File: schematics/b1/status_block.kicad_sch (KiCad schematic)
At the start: 22 parts, among them Q1 2N3904, SW5 SW_SPDT, U4 74HC595

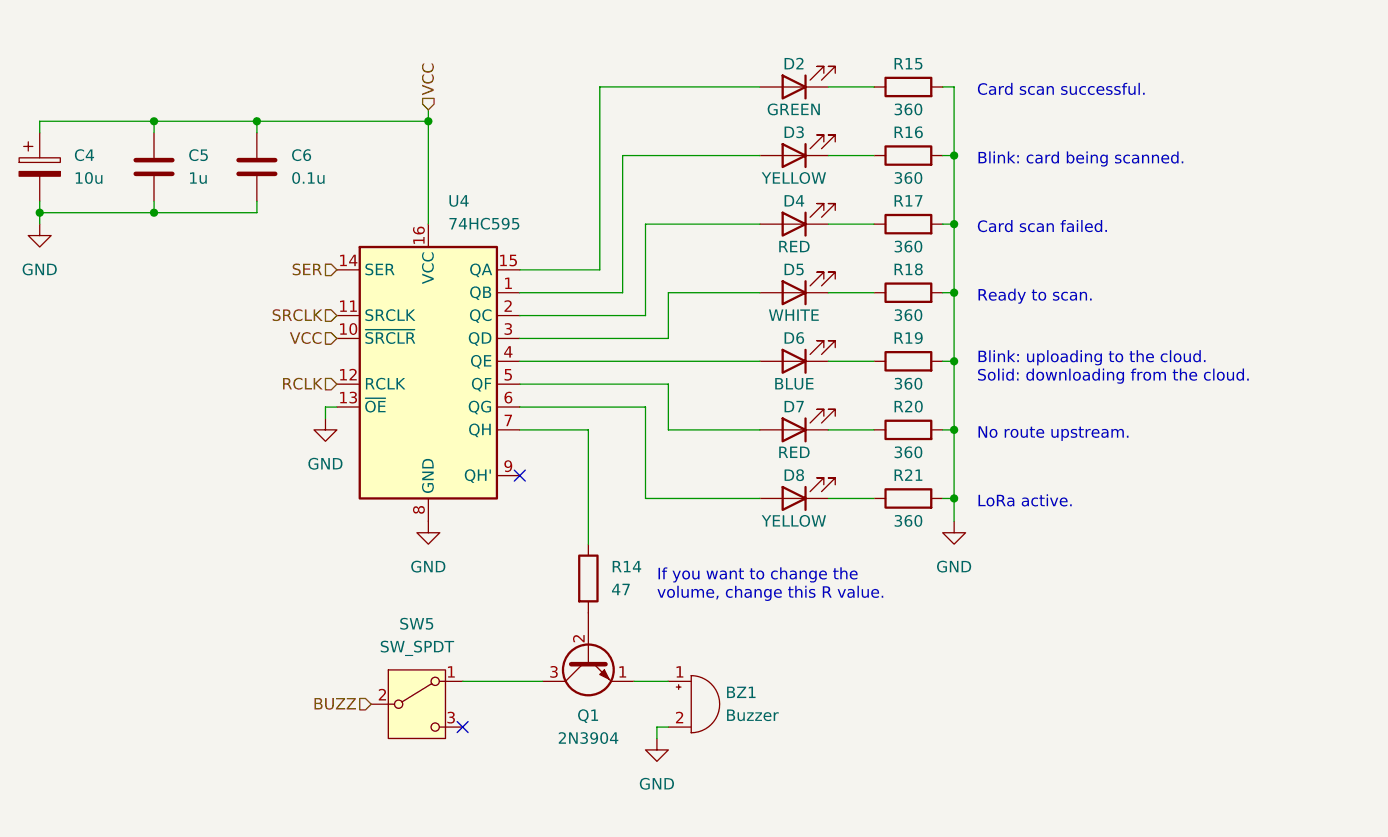
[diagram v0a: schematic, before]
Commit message: Updated buzz switch.
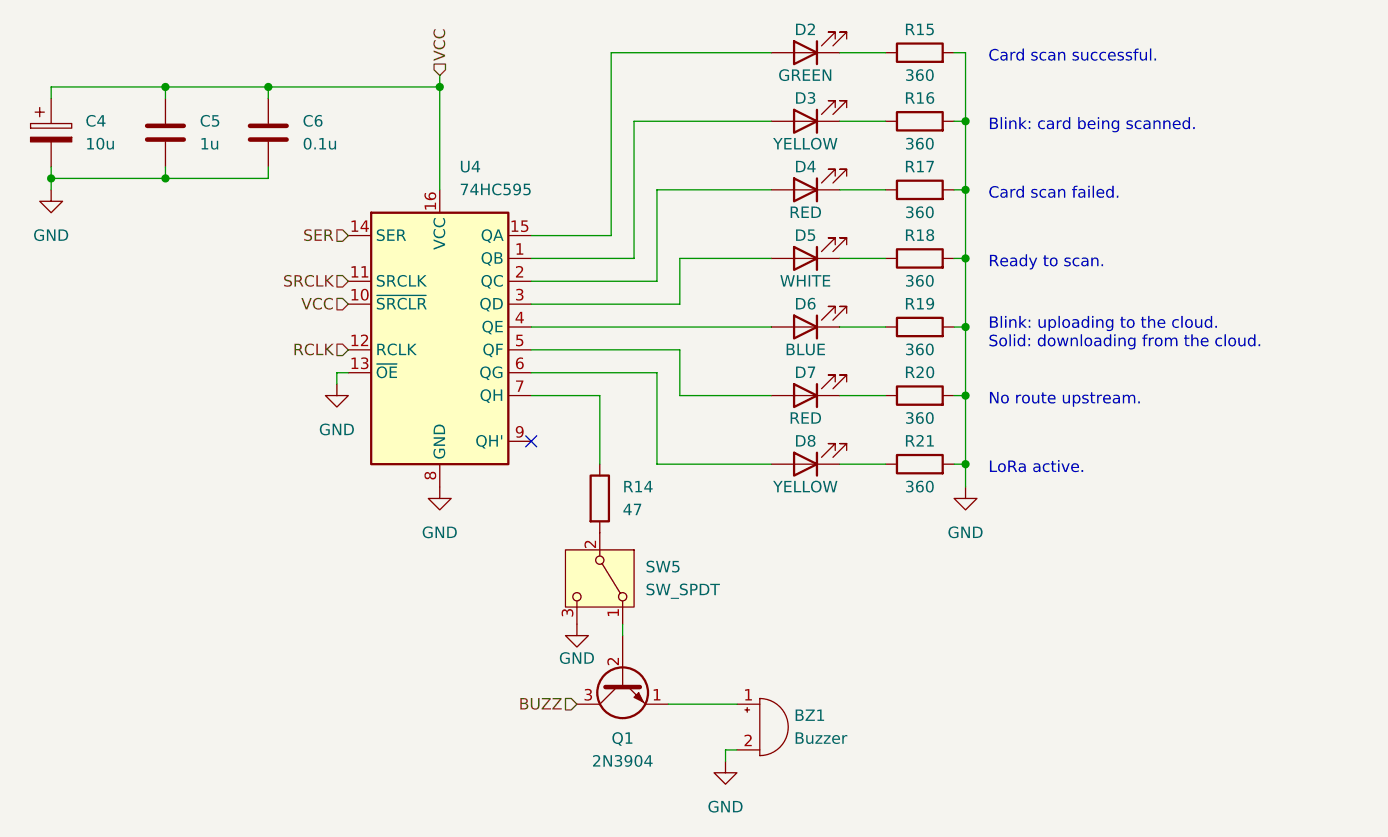
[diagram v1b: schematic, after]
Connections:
- net BUZZ: now also Q1.3 (C); no longer SW5.2 (B)
- net GND: now also SW5.3 (C)
- net at Q1.2 (B): now also SW5.1 (A); no longer R14.2
- new net: R14.2, SW5.2 (B)
- no-connect marks 2 -> 1
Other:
- note removed: "If you want to change the volume, change this R value."
- moved on the sheet: BZ1, C4, C5, C6, D2, D3, D4, D5, D6, D7, D8, Q1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
